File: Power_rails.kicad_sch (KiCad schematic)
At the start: 109 parts, among them Q1 SOC2222AHRG, Q2 SOC2222AHRG, U10 MAX8556ETE, U8 MAX8556ETE, U9 MAX8556ETE

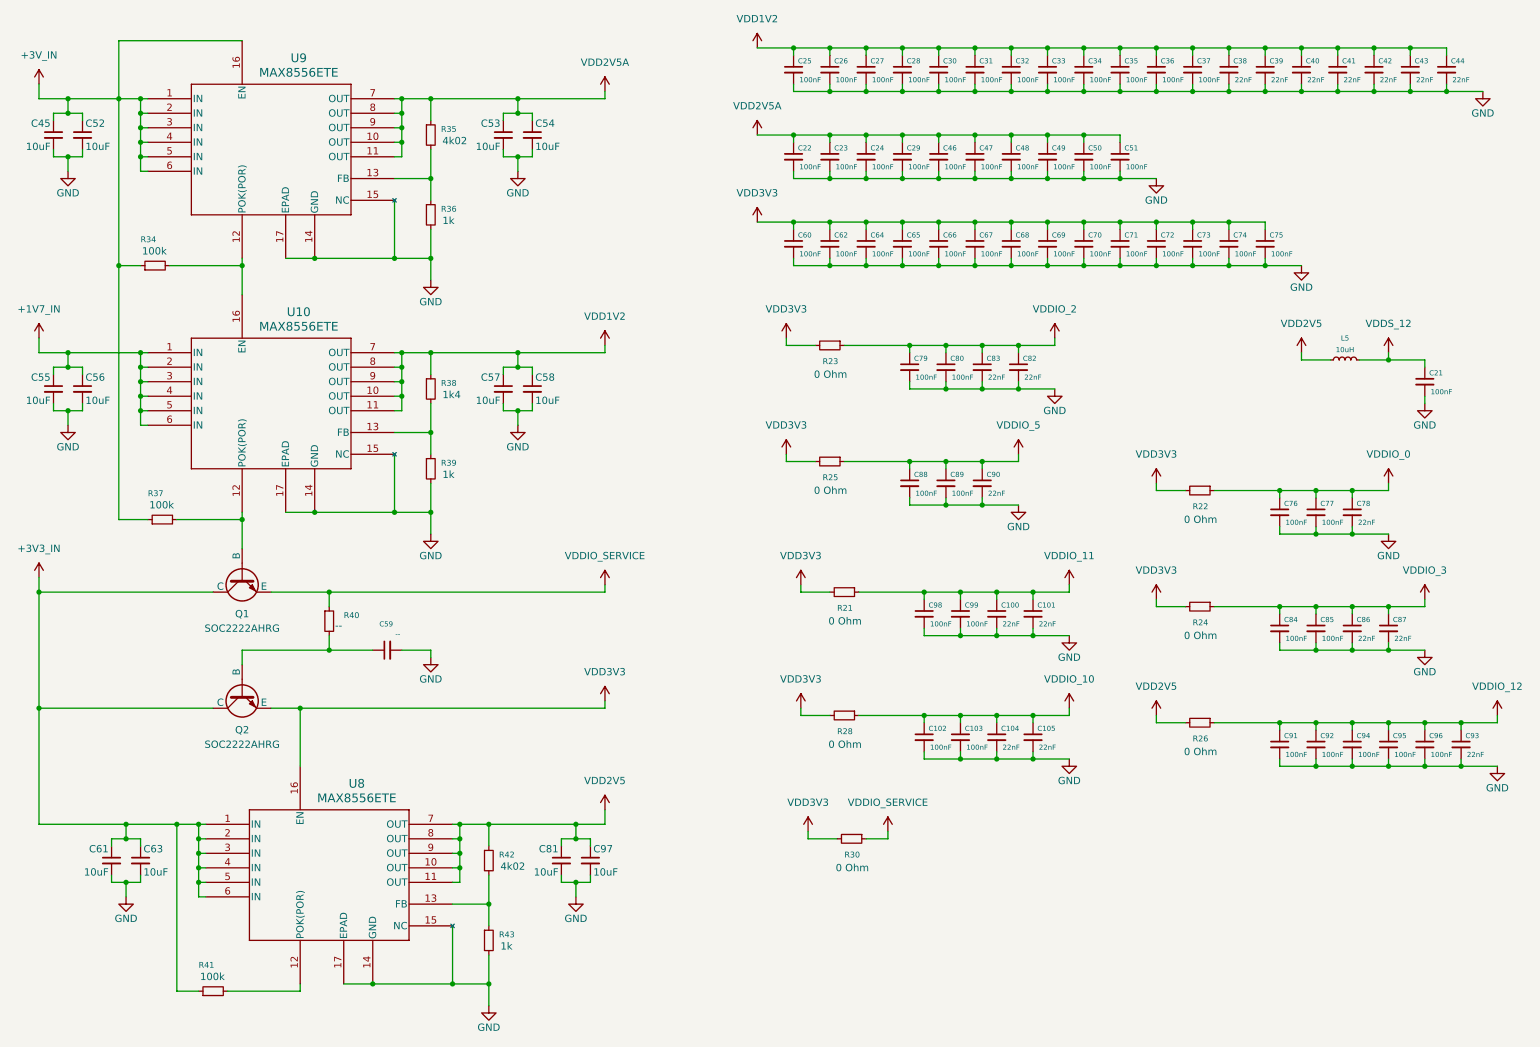
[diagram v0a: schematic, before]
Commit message: power tree
power tree defined. Few changes remaining but almost finalized
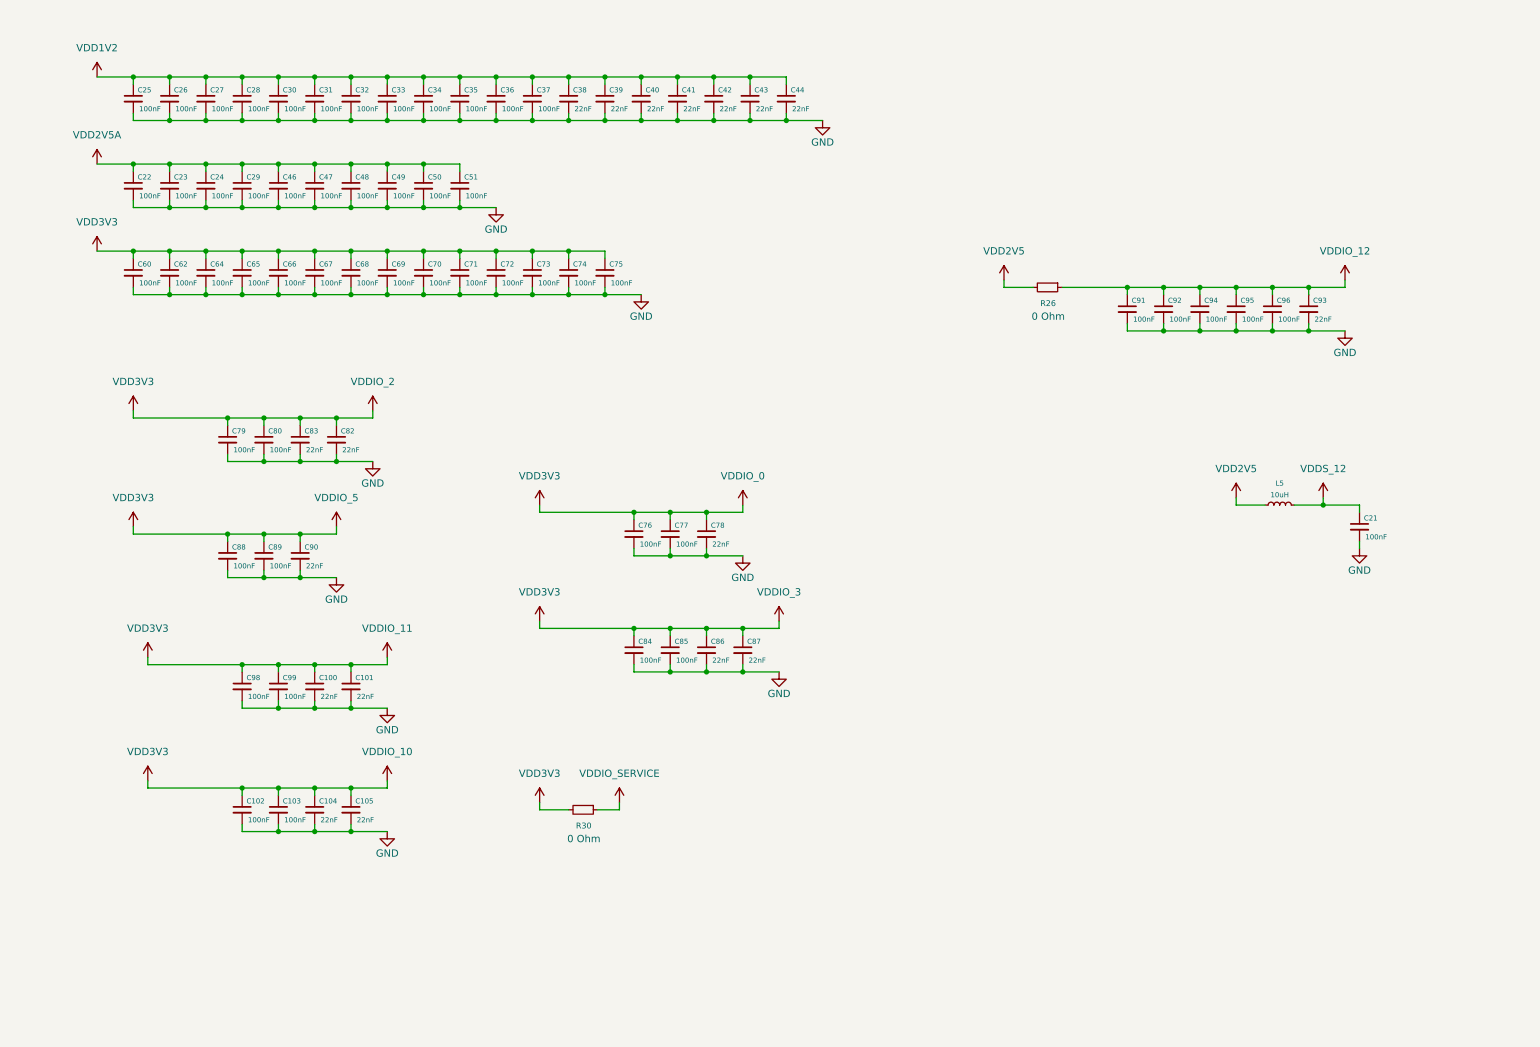
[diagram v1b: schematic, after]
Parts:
- removed C45, C52, C53, C54, C55, C56, C57, C58, C61, C63, C81, C97: 10uF, Capacitor_SMD:C_0603_1608Metric_Pad1.08x0.95mm_HandSolder, symbol Device:C_Small
- removed C59: --, Capacitor_SMD:C_0402_1005Metric_Pad0.74x0.62mm_HandSolder, symbol Device:C_Small
- removed Q1, Q2: SOC2222AHRG, DataHub_Footprints:NPN_LCC-3_STM, symbol Simulation_SPICE:NPN
- removed R21, R22, R23, R24, R25, R28: 0 Ohm, Resistor_SMD:R_0402_1005Metric_Pad0.72x0.64mm_HandSolder, symbol Device:R_Small
- removed R34, R37, R41: 100k, Resistor_SMD:R_0402_1005Metric_Pad0.72x0.64mm_HandSolder, symbol Device:R_Small
- removed R35, R42: 4k02, Resistor_SMD:R_0402_1005Metric_Pad0.72x0.64mm_HandSolder, symbol Device:R_Small
- removed R36, R39, R43: 1k, Resistor_SMD:R_0402_1005Metric_Pad0.72x0.64mm_HandSolder, symbol Device:R_Small
- removed R38: 1k4, Resistor_SMD:R_0402_1005Metric_Pad0.72x0.64mm_HandSolder, symbol Device:R_Small
- removed R40: --, Resistor_SMD:R_0402_1005Metric_Pad0.72x0.64mm_HandSolder, symbol Device:R_Small
- removed U10, U8, U9: MAX8556ETE, DataHub_Footprints:MAX8556, symbol MAX_LDO:MAX8556ETE
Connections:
- net VDDIO_0 is gone; now on net VDD3V3: C76.1, C77.1, C78.1
- net VDDIO_10 is gone; now on net VDD3V3: C102.1, C103.1, C104.1, C105.1
- net VDDIO_11 is gone; now on net VDD3V3: C100.1, C101.1, C98.1, C99.1
- net VDDIO_2 is gone; now on net VDD3V3: C79.1, C80.1, C82.1, C83.1
- net VDDIO_3 is gone; now on net VDD3V3: C84.1, C85.1, C86.1, C87.1
- net VDDIO_5 is gone; now on net VDD3V3: C88.1, C89.1, C90.1
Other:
- moved on the sheet: C100, C101, C102, C103, C104, C105, C21, C22, C23, C24, C25, C26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
